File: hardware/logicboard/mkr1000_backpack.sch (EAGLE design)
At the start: 12 parts, among them J3 3.3V, J4 DNP, J5 DNP

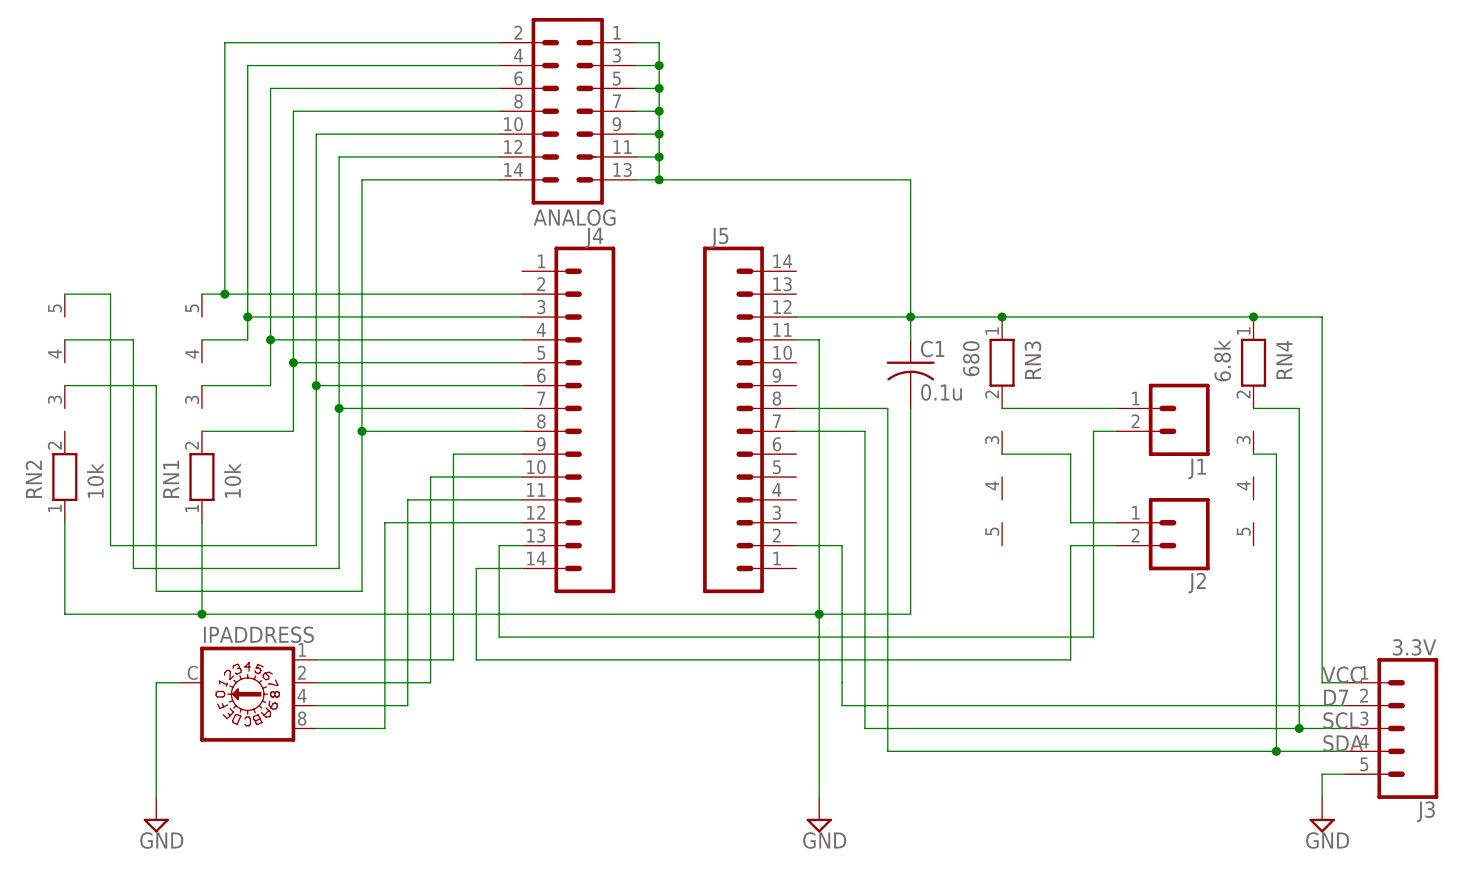
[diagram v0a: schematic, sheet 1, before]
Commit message: SparkFun Triple Axis Accelerometer Breakout - H3LIS331DL Ready.
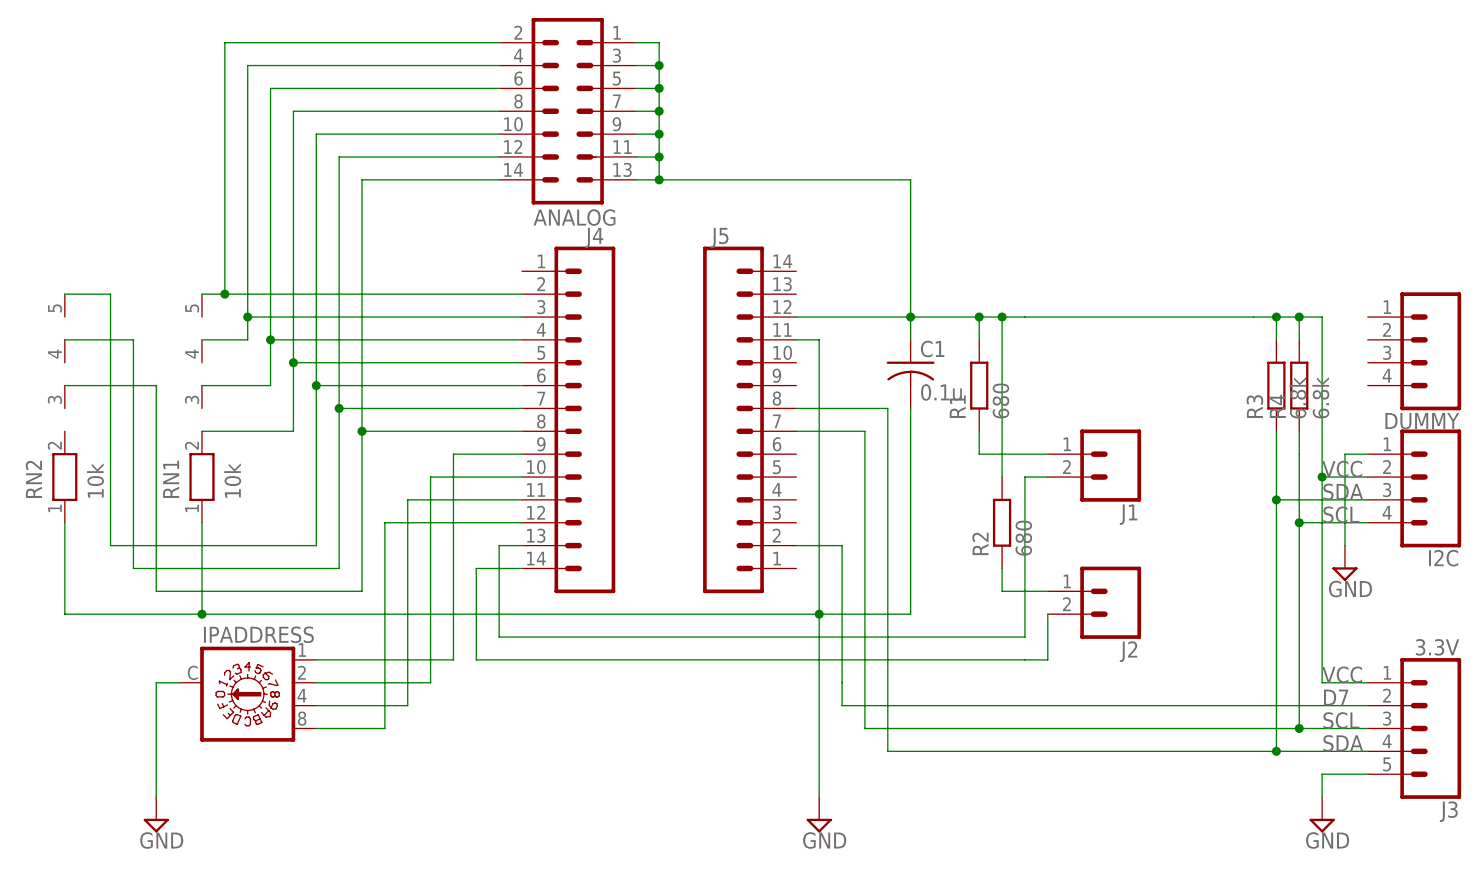
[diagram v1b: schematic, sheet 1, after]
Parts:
- removed RN3: 680, resistor-net:RN04
- removed RN4: 6.8k, resistor-net:RN04
- added DUMMY, I2C: (no value), SparkFun-Connectors:CONN_04
- added R1, R2: 680, resistor:R-EU_0204/5
- added R3, R4: 6.8k, resistor:R-EU_0204/5
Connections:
- net GND: now also I2C.1
- net N$1: now also R1.1; no longer RN3.2
- net N$2: now also R2.1; no longer RN3.3
- net SCL: now also I2C.4, R4.1; no longer RN4.2
- net SDA: now also I2C.3, R3.1; no longer RN4.3
- net VCC: now also I2C.2, R1.2, R2.2, R3.2, R4.2; no longer RN3.1, RN4.1
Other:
- moved on the sheet: J1, J2, J3
